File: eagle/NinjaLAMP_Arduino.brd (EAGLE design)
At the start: 50.8 x 33 mm, 13 parts

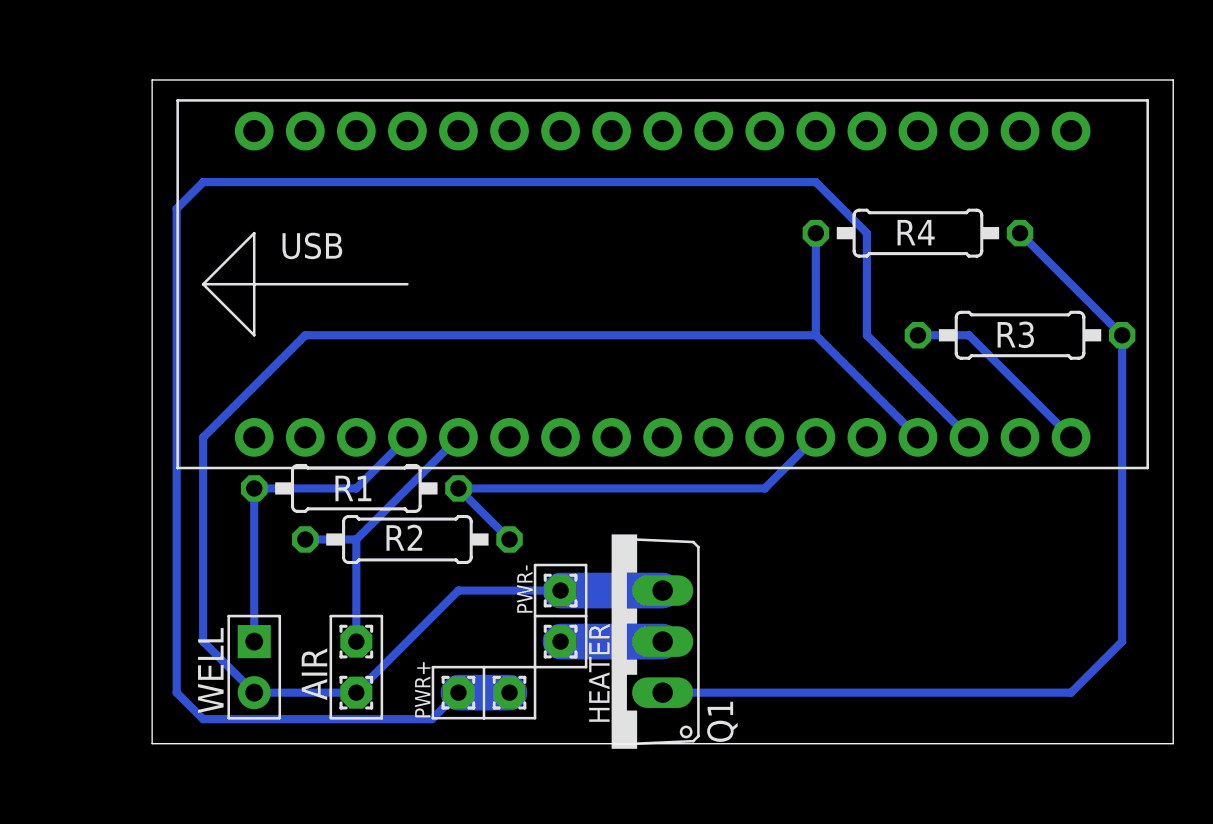
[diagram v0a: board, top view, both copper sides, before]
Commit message: t5.5 lasercut design finished
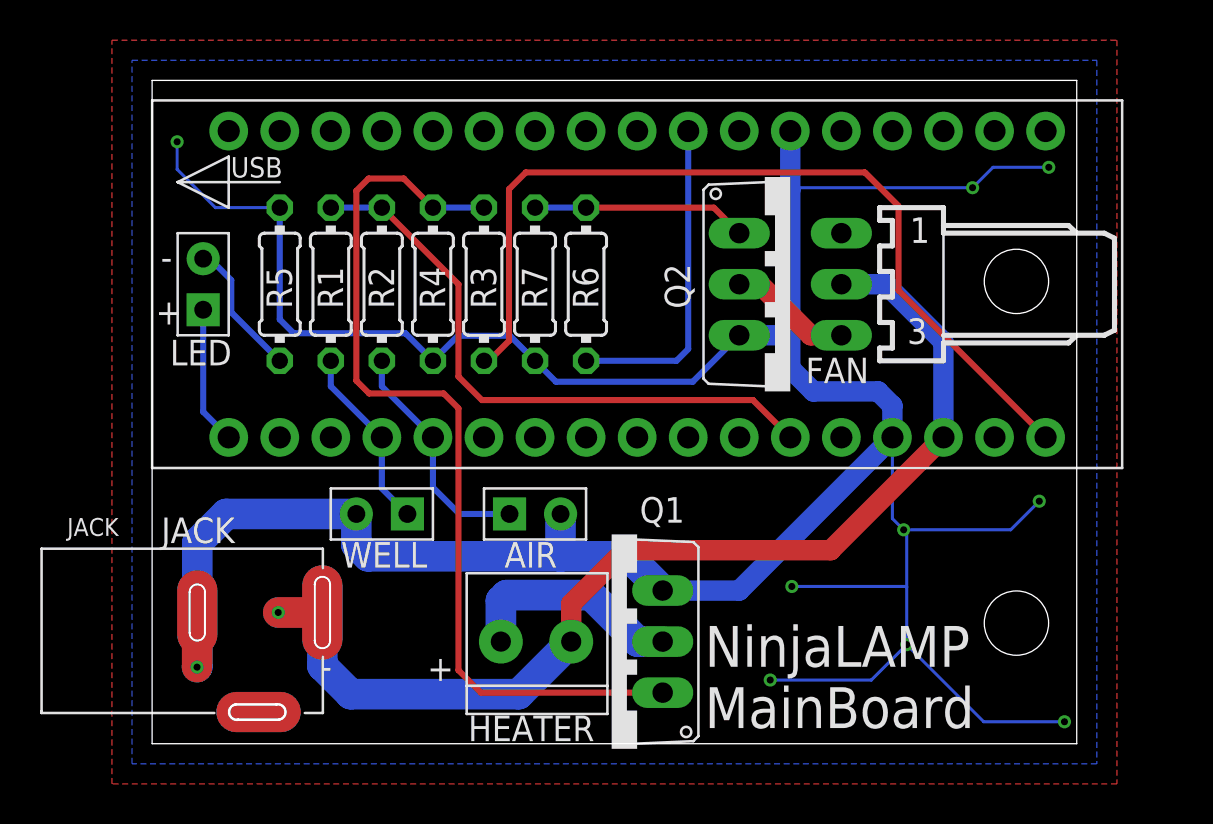
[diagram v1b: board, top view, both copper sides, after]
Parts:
- removed HEATER1, HEATER2, NTC_AIR1, NTC_AIR2, POWER+, POWER-: (no value), wirepad:1,6/0,8
- removed U$1: ARDUINOMICRO, adafruit:ARDUINOMICRO
- added HEATER: 1X2-3.5MM, adafruit:1X2-3.5MM
- added J1: 22-05-7038-03, con-molex:7395-03
- added JACK: DC-005, OPL_Connector:DCJ3P-14.2X11.0X9.0MM
- added LED, NTC_AIR: 2p-2.54, OPL_Connector:H2-2.54
- added Q2: (no value), adafruit:TO220V
- added R5, R6: 1K, resistor:0204/7
- added R7: 47K, resistor:0204/7
- added U$2: ARDUINOMICRO, adafruit:ARDUINOMICRO
- R1, R2, R3, R4: device resistor:0207/10 -> resistor:0204/7
- moved R3 26.8 mm to (16.5, 22.9), turned to 90 degrees
- moved R4 24.3 mm to (14.0, 22.9), turned to 270 degrees
- moved R2 12.8 mm to (11.4, 22.9), turned to 90 degrees
- moved R1 10.2 mm to (8.89, 22.9), turned to 90 degrees
- moved NTC_WELL 9.92 mm to (11.4, 11.4), turned to 270 degrees
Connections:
- new net D13: LED.1, U$2.P$34
- new net D3: R6.1, U$2.P$10
- new net N$2: LED.2, R5.2
- new net N$3: Q2.1, R6.2, R7.1
- new net N$6: J1.3, Q2.2
- net 12V: now also HEATER.1, J1.2, JACK.+B, JACK.+T, U$2.P$20; no longer HEATER1.1, POWER+.1, U$1.P$20
- net 5V: now also U$2.P$23; no longer U$1.P$23
- net A0: now also U$2.P$31; no longer U$1.P$31
- net A1: now also NTC_AIR.1, U$2.P$30; no longer NTC_AIR1.1, U$1.P$30
- net D15: now also U$2.P$18; no longer U$1.P$18
- net DRAIN: now also HEATER.2; no longer HEATER2.1
- net GND: now also JACK.-1B, JACK.-1T, NTC_AIR.2, Q2.3, R5.1, R7.2, U$2.P$12, U$2.P$21; no longer NTC_AIR2.1, POWER-.1, U$1.P$12
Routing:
- net GND: track 81.0 -> 167.1 mm, vias 0 -> 10
- net D15: track 9.72 -> 44.2 mm
- net 12V: track 89.9 -> 55.9 mm, vias 0 -> 1
- net D3: track 0.00 -> 16.2 mm
- net N$3: track 0.00 -> 10.7 mm
- net 5V: track 22.4 -> 30.3 mm
- net A0: track 16.3 -> 9.20 mm
- net D13: track 0.00 -> 6.88 mm
- net N$2: track 0.00 -> 6.85 mm
- net N$6: track 0.00 -> 6.13 mm
- net DRAIN: track 5.08 -> 11.2 mm
- net A1: track 14.8 -> 11.7 mm
- added copper zone on layer 1, net GND
- added copper zone on layer 16, net GND
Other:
- board size 50.8 x 33 mm -> 46 x 33 mm
- board text added: "+"
- board text added: "-"
- board text added: "FAN"
- board text added: "JACK"
- board text added: "LED"
- board text added: "NinjaLAMP MainBoard"
- board text added: "Q1"
- board text added: "Q2"
- board text added: "R1"
- board text added: "R2"
- board text added: "R3"
- board text added: "R4"
- board text added: "R5"
- board text added: "R6"
- board text added: "R7"
- board text removed: "PWR+"
- board text removed: "PWR-"
